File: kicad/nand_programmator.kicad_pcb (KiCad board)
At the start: 2 copper layers, 48 x 41 mm, 42 parts, among them J1 Conn_01x04, J2 Conn_01x03, J3 Conn_02x12_Odd_Even_Left, J4 Conn_02x12_Odd_Even_Right, J5 BOOT0, J6 ~{RST}, P1 USB, U1 LM1117-3.3, U2 STM32F103VCT6, Y1 Crystal_SMD_8MHz_18pF

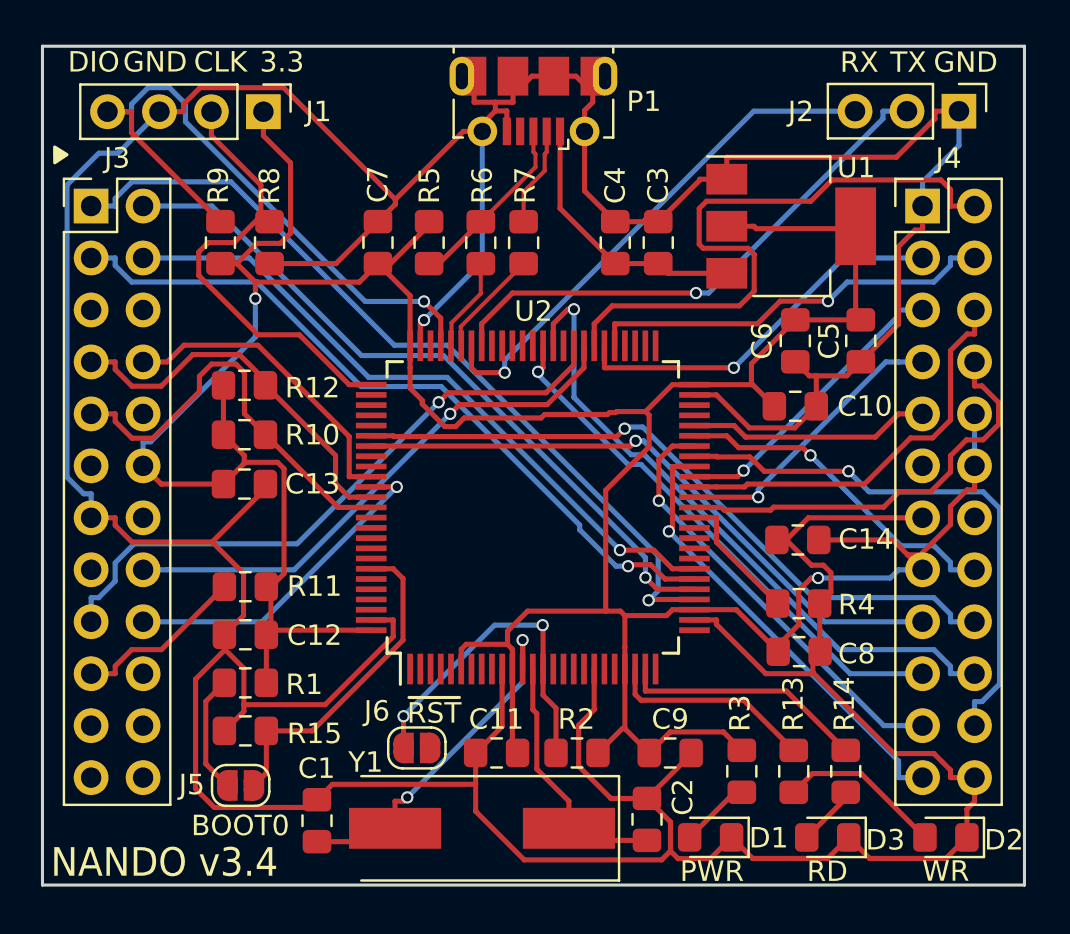
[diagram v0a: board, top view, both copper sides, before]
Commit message: update PCB design and cleanup KiCad files
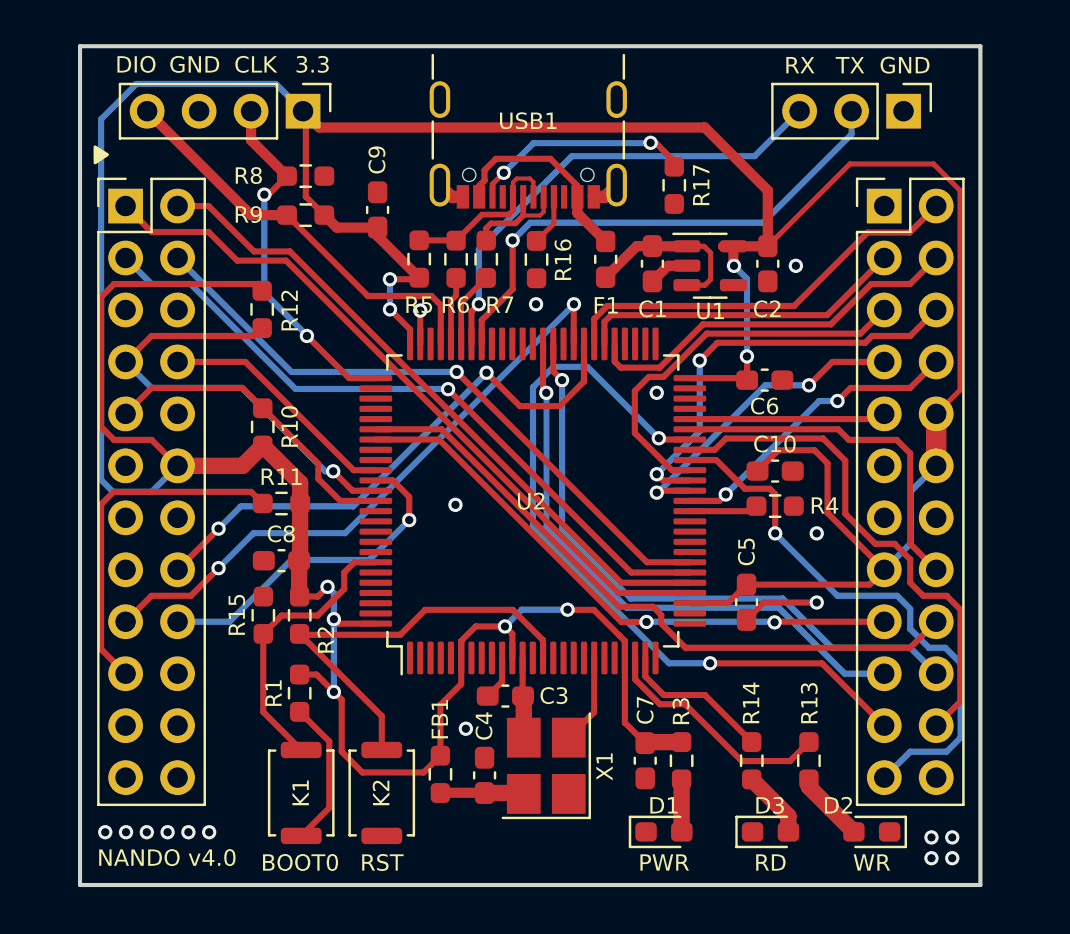
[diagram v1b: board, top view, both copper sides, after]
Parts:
- removed the C1 at (181.3, 82.5)
- removed the C2 at (197.4, 82.4)
- removed the C5 at (207.9, 59.0)
- removed the C7 at (184.3, 54.2)
- removed the C8 at (204.9, 74.2)
- removed P1: USB, lib_fp:USB_Micro-B_Molex-105017-0001
- removed Y1: Crystal_SMD_8MHz_18pF, lib_fp:Crystal_SMD_HC49-SD
- added C3: 15pF, Capacitor_SMD:C_0603_1608Metric_Pad1.08x0.95mm_HandSolder, F.Cu at (190.5, 76.4)
- added F1: 500mA, 6V, Fuse:Fuse_0603_1608Metric_Pad1.05x0.95mm_HandSolder, F.Cu at (195.4, 55.1)
- added FB1: FerriteBead_600Ω@100MHz, Resistor_SMD:R_0603_1608Metric_Pad0.98x0.95mm_HandSolder, F.Cu at (187.3, 80.2)
- added R16: 5.1K, Resistor_SMD:R_0603_1608Metric_Pad0.98x0.95mm_HandSolder, F.Cu at (192.0, 55.1)
- added R17: 5.1K, Resistor_SMD:R_0603_1608Metric_Pad0.98x0.95mm_HandSolder, F.Cu at (198.8, 51.4)
- added USB1: USB_C_Receptacle_USB2.0, Connector_USB:USB_C_Receptacle_GCT_USB4105-xx-A_16P_TopMnt_Horizontal, F.Cu at (191.6, 48.3)
- added X1: 8MHz 3.3V, Oscillator:Oscillator_SMD_Abracon_ASE-4Pin_3.2x2.5mm_HandSoldering, F.Cu at (192.5, 79.8)
- C1: renamed from C3; value 10uF -> 1uF; footprint lib_fp:C_0805_2012Metric_Pad1.15x1.40mm_HandSolder -> Capacitor_SMD:C_0603_1608Metric_Pad1.08x0.95mm_HandSolder
- C10: renamed from C14; footprint lib_fp:C_0805_2012Metric_Pad1.15x1.40mm_HandSolder -> Capacitor_SMD:C_0603_1608Metric_Pad1.08x0.95mm_HandSolder
- C2: renamed from C6; value 10uF -> 1uF; footprint lib_fp:C_0805_2012Metric_Pad1.15x1.40mm_HandSolder -> Capacitor_SMD:C_0603_1608Metric_Pad1.08x0.95mm_HandSolder
- C4: footprint lib_fp:C_0805_2012Metric_Pad1.15x1.40mm_HandSolder -> Capacitor_SMD:C_0603_1608Metric_Pad1.08x0.95mm_HandSolder
- C5: renamed from C9; footprint lib_fp:C_0805_2012Metric_Pad1.15x1.40mm_HandSolder -> Capacitor_SMD:C_0603_1608Metric_Pad1.08x0.95mm_HandSolder
- C6: renamed from C10; footprint lib_fp:C_0805_2012Metric_Pad1.15x1.40mm_HandSolder -> Capacitor_SMD:C_0603_1608Metric_Pad1.08x0.95mm_HandSolder
- C7: renamed from C11; footprint lib_fp:C_0805_2012Metric_Pad1.15x1.40mm_HandSolder -> Capacitor_SMD:C_0603_1608Metric_Pad1.08x0.95mm_HandSolder
- C8: renamed from C12; footprint lib_fp:C_0805_2012Metric_Pad1.15x1.40mm_HandSolder -> Capacitor_SMD:C_0603_1608Metric_Pad1.08x0.95mm_HandSolder
- C9: renamed from C13; footprint lib_fp:C_0805_2012Metric_Pad1.15x1.40mm_HandSolder -> Capacitor_SMD:C_0603_1608Metric_Pad1.08x0.95mm_HandSolder
- D1, D2, D3: footprint lib_fp:LED_0805_2012Metric_Pad1.15x1.40mm_HandSolder -> LED_SMD:LED_0603_1608Metric_Pad1.05x0.95mm_HandSolder
- J1: footprint lib_fp:PinHeader_1x04_P2.54mm_Vertical -> Connector_PinHeader_2.54mm:PinHeader_1x04_P2.54mm_Vertical
- J2: footprint lib_fp:PinHeader_1x03_P2.54mm_Vertical -> Connector_PinHeader_2.54mm:PinHeader_1x03_P2.54mm_Vertical
- J3: footprint lib_fp:PinHeader_2x12_P2.54mm_Vertical -> Connector_PinHeader_2.54mm:PinHeader_2x12_P2.54mm_Vertical
- K1: renamed from J5; footprint lib_fp:SolderJumper-2_P1.3mm_Open_RoundedPad1.0x1.5mm -> Button_Switch_SMD:SW_Push_SPST_NO_Alps_SKRK
- K2: renamed from J6; value ~{RST} -> ~RST; footprint lib_fp:SolderJumper-2_P1.3mm_Open_RoundedPad1.0x1.5mm -> Button_Switch_SMD:SW_Push_SPST_NO_Alps_SKRK
- R1, R10, R11, R12, R15, R2, R4, R5, R6, R7, R8, R9: footprint lib_fp:R_0805_2012Metric_Pad1.15x1.40mm_HandSolder -> Resistor_SMD:R_0603_1608Metric_Pad0.98x0.95mm_HandSolder
- R13, R14: value 1k -> 2.2k; footprint lib_fp:R_0805_2012Metric_Pad1.15x1.40mm_HandSolder -> Resistor_SMD:R_0603_1608Metric_Pad0.98x0.95mm_HandSolder
- R3: value 1k -> 4.7k; footprint lib_fp:R_0805_2012Metric_Pad1.15x1.40mm_HandSolder -> Resistor_SMD:R_0603_1608Metric_Pad0.98x0.95mm_HandSolder
- U1: value LM1117-3.3 -> RT9013-33GB; footprint lib_fp:SOT-223 -> Package_TO_SOT_SMD:SOT-23-5
- U2: footprint lib_fp:LQFP-100_14x14mm_Pitch0.5mm -> Package_QFP:LQFP-100_14x14mm_P0.5mm
- moved C4 26.8 mm to (189.5, 80.3)
- moved R2 15.1 mm to (180.4, 72.5), turned to -90 degrees
- moved C9 14.9 mm to (184.3, 52.6), turned to -90 degrees
- moved C5 8.26 mm to (202.3, 71.8), turned to -90 degrees
- moved C7 7.27 mm to (197.3, 79.6), turned to -90 degrees
- moved R15 5.72 mm to (178.7, 72.5), turned to -90 degrees
- moved R4 4.90 mm to (203.7, 67.1)
- moved R14 4.62 mm to (202.5, 79.6)
- moved R11 4.43 mm to (179.6, 67.0)
- moved U1 4.41 mm to (200.5, 55.4)
- moved R9 4.38 mm to (180.7, 52.9), turned to 180 degrees
- moved C8 4.03 mm to (179.6, 69.8)
- moved C2 4.00 mm to (203.3, 55.3)
- moved R12 3.81 mm to (178.6, 57.5), turned to -90 degrees
- moved R8 3.70 mm to (180.7, 51.0), turned to 180 degrees
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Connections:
- C4 pad 1: +5V -> Net-(X1-VDD)
- J3 pad 10: Net-(J3-Pad10) -> unconnected-(J3-Pin_10-Pad10)
- J3 pad 11: Net-(J3-Pad11) -> unconnected-(J3-Pin_11-Pad11)
- J3 pad 14: Net-(J3-Pad14) -> unconnected-(J3-Pin_14-Pad14)
- J3 pad 15: Net-(J3-Pad15) -> unconnected-(J3-Pin_15-Pad15)
- J3 pad 20: Net-(J3-Pad20) -> unconnected-(J3-Pin_20-Pad20)
- J3 pad 21: Net-(J3-Pad21) -> unconnected-(J3-Pin_21-Pad21)
- J3 pad 22: Net-(J3-Pad22) -> unconnected-(J3-Pin_22-Pad22)
- J3 pad 23: Net-(J3-Pad23) -> unconnected-(J3-Pin_23-Pad23)
- J3 pad 24: Net-(J3-Pad24) -> unconnected-(J3-Pin_24-Pad24)
- J3 pad 5: Net-(J3-Pad5) -> unconnected-(J3-Pin_5-Pad5)
- J3 pad 6: Net-(J3-Pad6) -> unconnected-(J3-Pin_6-Pad6)
- J4 pad 35: Net-(J4-Pad35) -> unconnected-(J4-Pin_35-Pad35)
- J4 pad 38: Net-(J4-Pad38) -> unconnected-(J4-Pin_38-Pad38)
- R5 pad 1: /USB_P -> +3V3
- R5 pad 2: +3V3 -> /USB_P
- R6 pad 1: /USB_DP -> /USB_P
- R6 pad 2: /USB_P -> /USB_DP
- U1 pad 1: GNDD -> +5V
- U1 pad 2: +3V3 -> GNDD
- U1 pad 4: +3V3 -> unconnected-(U1-NC-Pad4)
- U2 pad 1: Net-(U2-Pad1) -> unconnected-(U2-PE2/FSMC_A23/SYS_TRACECLK-Pad1)
- U2 pad 13: Net-(C2-Pad1) -> unconnected-(U2-RCC_OSC_OUT-Pad13)
- U2 pad 15: Net-(U2-Pad15) -> unconnected-(U2-ADC1_IN10/ADC2_IN10/ADC3_IN10/PC0-Pad15)
- U2 pad 16: Net-(U2-Pad16) -> unconnected-(U2-ADC1_IN11/ADC2_IN11/ADC3_IN11/PC1-Pad16)
- U2 pad 17: Net-(U2-Pad17) -> unconnected-(U2-ADC1_IN12/ADC2_IN12/ADC3_IN12/PC2-Pad17)
- U2 pad 18: Net-(U2-Pad18) -> unconnected-(U2-ADC1_IN13/ADC2_IN13/ADC3_IN13/PC3-Pad18)
- U2 pad 2: Net-(U2-Pad2) -> unconnected-(U2-PE3/FSMC_A19/SYS_TRACED0-Pad2)
- U2 pad 20: Net-(U2-Pad20) -> unconnected-(U2-VREF--Pad20)
- U2 pad 21: Net-(U2-Pad21) -> unconnected-(U2-VREF+-Pad21)
- U2 pad 25: Net-(U2-Pad25) -> unconnected-(U2-ADC1_IN2/ADC2_IN2/ADC3_IN2/TIM2_CH3/TIM5_CH3/USART2_TX/PA2-Pad25)
- U2 pad 26: Net-(U2-Pad26) -> unconnected-(U2-ADC1_IN3/ADC2_IN3/ADC3_IN3/TIM2_CH4/TIM5_CH4/USART2_RX/PA3-Pad26)
- U2 pad 3: Net-(U2-Pad3) -> unconnected-(U2-PE4/FSMC_A20/SYS_TRACED1-Pad3)
- U2 pad 33: Net-(U2-Pad33) -> unconnected-(U2-ADC1_IN14/ADC2_IN14/PC4-Pad33)
- U2 pad 34: Net-(U2-Pad34) -> unconnected-(U2-ADC1_IN15/ADC2_IN15/PC5-Pad34)
- U2 pad 35: Net-(U2-Pad35) -> unconnected-(U2-ADC1_IN8/ADC2_IN8/TIM1_CH2N/TIM3_CH3/TIM8_CH2N/PB0-Pad35)
- U2 pad 36: Net-(U2-Pad36) -> unconnected-(U2-ADC1_IN9/ADC2_IN9/TIM1_CH3N/TIM3_CH4/TIM8_CH3N/PB1-Pad36)
- U2 pad 4: Net-(U2-Pad4) -> unconnected-(U2-PE5/FSMC_A21/SYS_TRACED2-Pad4)
- U2 pad 47: Net-(U2-Pad47) -> unconnected-(U2-I2C2_SCL/TIM2_CH3/USART3_TX/PB10-Pad47)
- U2 pad 48: Net-(U2-Pad48) -> unconnected-(U2-ADC1_EXTI11/ADC2_EXTI11/I2C2_SDA/TIM2_CH4/USART3_RX/PB11-Pad48)
- U2 pad 5: Net-(U2-Pad5) -> unconnected-(U2-PE6/FSMC_A22/SYS_TRACED3-Pad5)
- U2 pad 51: Net-(U2-Pad51) -> unconnected-(U2-I2C2_SMBA/I2S2_WS/SPI2_NSS/TIM1_BKIN/USART3_CK/PB12-Pad51)
- U2 pad 52: Net-(U2-Pad52) -> unconnected-(U2-I2S2_CK/SPI2_SCK/TIM1_CH1N/USART3_CTS/PB13-Pad52)
- U2 pad 53: Net-(U2-Pad53) -> unconnected-(U2-SPI2_MISO/TIM1_CH2N/USART3_RTS/PB14-Pad53)
- U2 pad 54: Net-(U2-Pad54) -> unconnected-(U2-ADC1_EXTI15/ADC2_EXTI15/I2S2_SD/SPI2_MOSI/TIM1_CH3N/PB15-Pad54)
- U2 pad 60: Net-(U2-Pad60) -> unconnected-(U2-PD13/FSMC_A18/TIM4_CH2-Pad60)
- U2 pad 63: Net-(U2-Pad63) -> unconnected-(U2-I2S2_MCK/SDIO_D6/TIM3_CH1/TIM8_CH1/PC6-Pad63)
- U2 pad 64: Net-(U2-Pad64) -> unconnected-(U2-I2S3_MCK/SDIO_D7/TIM3_CH2/TIM8_CH2/PC7-Pad64)
- U2 pad 65: Net-(U2-Pad65) -> unconnected-(U2-SDIO_D0/TIM3_CH3/TIM8_CH3/PC8-Pad65)
- U2 pad 66: Net-(U2-Pad66) -> unconnected-(U2-DAC_EXTI9/SDIO_D1/TIM3_CH4/TIM8_CH4/PC9-Pad66)
- U2 pad 67: Net-(U2-Pad67) -> unconnected-(U2-RCC_MCO/TIM1_CH1/USART1_CK/PA8-Pad67)
- U2 pad 7: Net-(U2-Pad7) -> unconnected-(U2-RTC_OUT/RTC_TAMPER/PC13-Pad7)
- U2 pad 73: Net-(U2-Pad73) -> unconnected-(U2-NC-Pad73)
- U2 pad 77: Net-(U2-Pad77) -> unconnected-(U2-ADC1_EXTI15/ADC2_EXTI15/I2S3_WS/SPI1_NSS/SPI3_NSS/SYS_JTDI/TIM2_CH1/TIM2_ETR/PA15-Pad77)
- U2 pad 78: Net-(U2-Pad78) -> unconnected-(U2-SDIO_D2/UART4_TX/USART3_TX/PC10-Pad78)
- U2 pad 79: Net-(U2-Pad79) -> unconnected-(U2-ADC1_EXTI11/ADC2_EXTI11/SDIO_D3/UART4_RX/USART3_RX/PC11-Pad79)
- U2 pad 8: Net-(U2-Pad8) -> unconnected-(U2-RCC_OSC32_IN/PC14-Pad8)
- U2 pad 80: Net-(U2-Pad80) -> unconnected-(U2-SDIO_CK/UART5_TX/USART3_CK/PC12-Pad80)
- U2 pad 83: Net-(U2-Pad83) -> unconnected-(U2-PD2/SDIO_CMD/TIM3_ETR/UART5_RX-Pad83)
- U2 pad 84: Net-(U2-Pad84) -> unconnected-(U2-PD3/FSMC_CLK/USART2_CTS-Pad84)
- U2 pad 89: Net-(U2-Pad89) -> unconnected-(U2-I2S3_CK/SPI1_SCK/SPI3_SCK/SYS_JTDO-TRACESWO/TIM2_CH2/PB3-Pad89)
- U2 pad 9: Net-(U2-Pad9) -> unconnected-(U2-ADC1_EXTI15/ADC2_EXTI15/RCC_OSC32_OUT/PC15-Pad9)
- U2 pad 90: Net-(U2-Pad90) -> unconnected-(U2-SPI1_MISO/SPI3_MISO/SYS_NJTRST/TIM3_CH1/PB4-Pad90)
- U2 pad 91: Net-(U2-Pad91) -> unconnected-(U2-I2C1_SMBA/I2S3_SD/SPI1_MOSI/SPI3_MOSI/TIM3_CH2/PB5-Pad91)
- U2 pad 92: Net-(U2-Pad92) -> unconnected-(U2-I2C1_SCL/TIM4_CH1/USART1_TX/PB6-Pad92)
- U2 pad 93: Net-(U2-Pad93) -> unconnected-(U2-FSMC_NL/I2C1_SDA/TIM4_CH2/USART1_RX/PB7-Pad93)
- U2 pad 95: Net-(U2-Pad95) -> unconnected-(U2-CAN_RX/I2C1_SCL/SDIO_D4/TIM4_CH3/PB8-Pad95)
- U2 pad 96: Net-(U2-Pad96) -> unconnected-(U2-CAN_TX/DAC_EXTI9/I2C1_SDA/SDIO_D5/TIM4_CH4/PB9-Pad96)
- U2 pad 97: Net-(U2-Pad97) -> unconnected-(U2-PE0/FSMC_NBL0/TIM4_ETR-Pad97)
- U2 pad 98: Net-(U2-Pad98) -> unconnected-(U2-PE1/FSMC_NBL1-Pad98)
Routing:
- net GNDD: track 270.6 -> 16.8 mm, vias 1 -> 18
- net +3V3: track 179.4 -> 216.8 mm, vias 2 -> 9
- net /FSMC_D10: track 21.5 -> 37.6 mm, vias 1 -> 2
- net Net-(U2-RCC_OSC_IN): track 17.5 -> 3.92 mm, vias 2 -> 0
- net Net-(C2-Pad1): track 12.6 -> 0.00 mm
- net /SWDIO: track 31.9 -> 20.2 mm, vias 1 -> 0
- net /FSMC_D15: track 31.0 -> 20.2 mm
- net Net-(USB1-CC2): track 0.00 -> 10.7 mm, vias 0 -> 2
- net Net-(F1-Pad1): track 0.00 -> 10.0 mm
- net Net-(J3-Pin_19): track 8.49 -> 17.2 mm
- net /FSMC_D4: track 20.9 -> 14.9 mm, vias 0 -> 2
- net /SPI1_NSS: track 40.6 -> 35.4 mm, vias 1 -> 0
- net /FSMC_D8: track 22.2 -> 27.2 mm
- net /FSMC_NCE2: track 20.4 -> 15.5 mm
- net /SWCLK: track 22.2 -> 17.4 mm, vias 0 -> 2
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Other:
- board size 48 x 41 mm -> 44 x 41 mm
- rule pad_to_mask_clearance: 0.2 -> 0.05
- rule solder_mask_min_width: 0.25 -> 0.1
- board text added: "NANDO v4.0"
- board text added: "RST"
- board text removed: "NANDO v3.4"
